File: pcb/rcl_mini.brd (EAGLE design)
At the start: 160 x 100 mm, 59 parts, among them CN1 USB mini B, Q1 8MHz, Q2 IRLML5203, U1 MCP6002T-I/SN, U2 MCP6002T-I/SN, U3 MCP6002T-I/SN, U4 STM32F100CBT6, U5 MCP73831/OT, U6 MCP1703CB, X1 BAT, X2 TWEEZERS, X3 OLED, X4 SWD

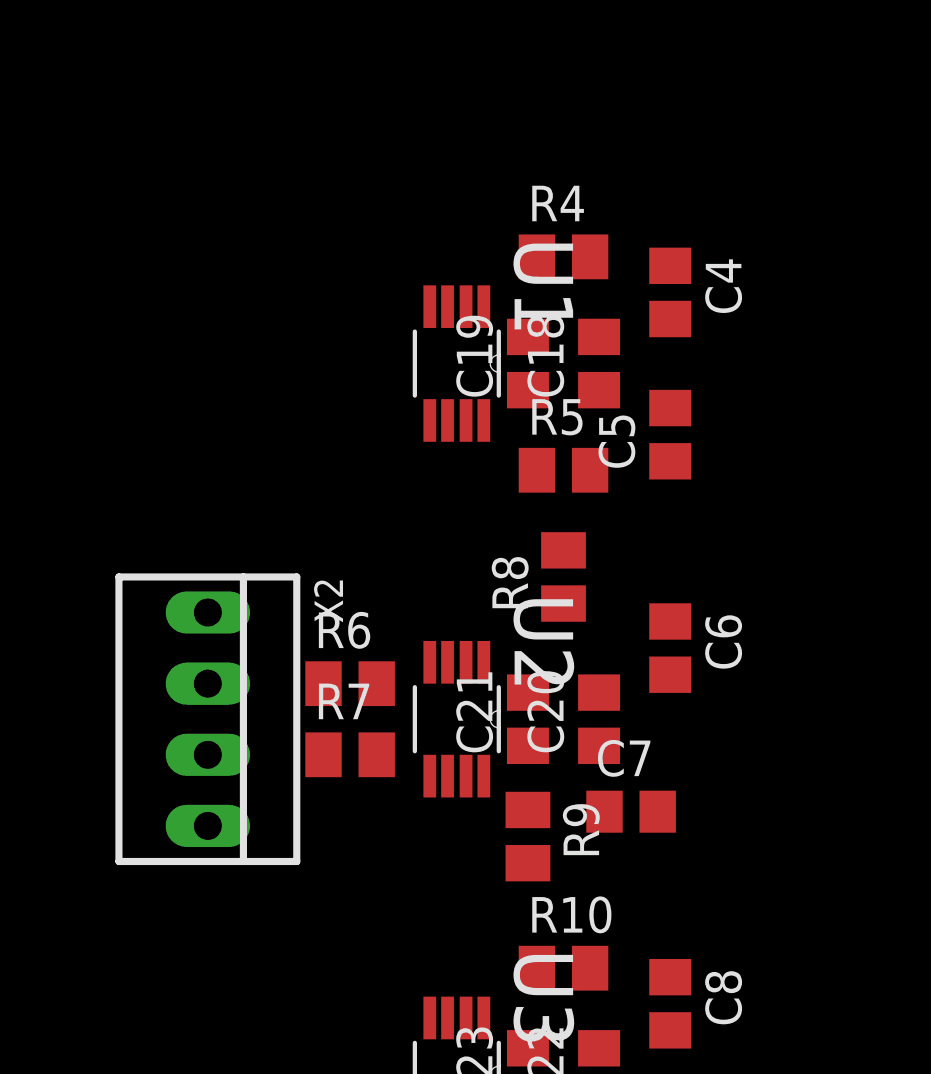
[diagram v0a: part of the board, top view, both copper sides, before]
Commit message: pcb v1.0
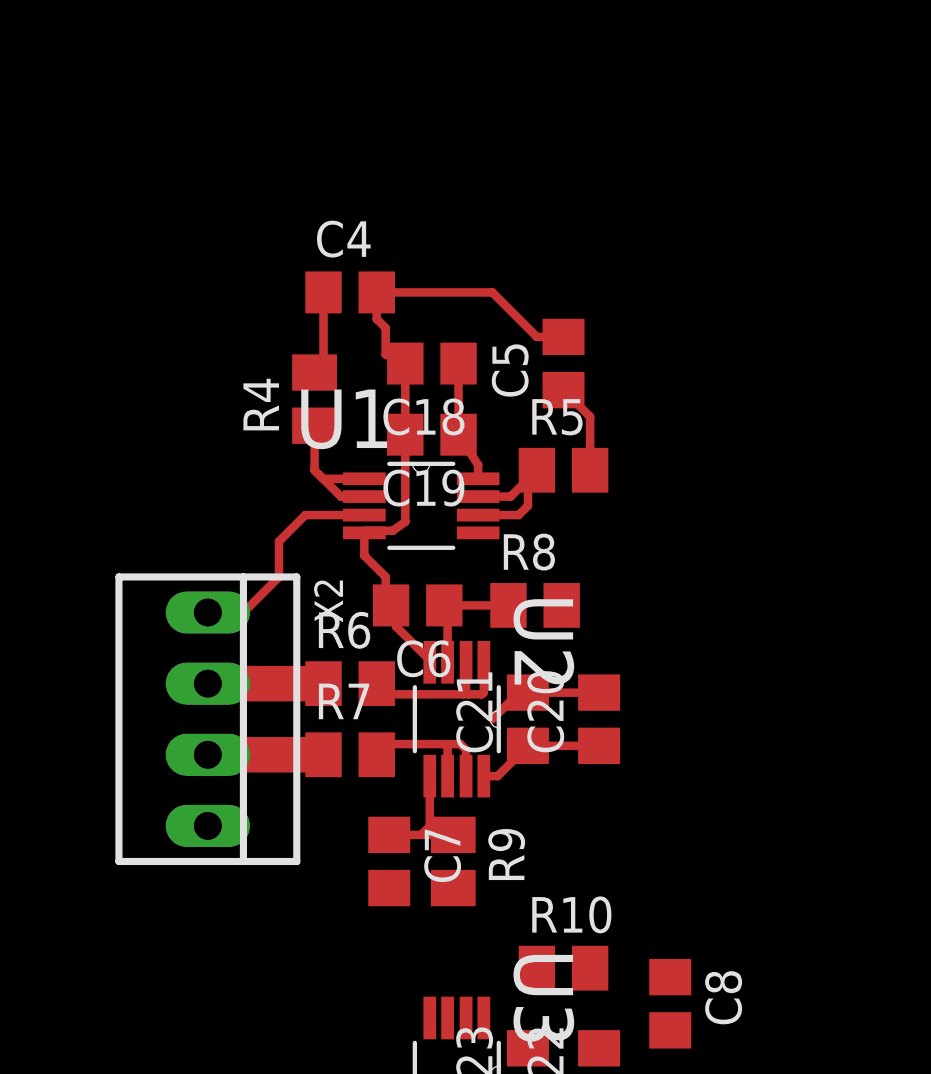
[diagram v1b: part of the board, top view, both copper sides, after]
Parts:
- moved C4 11.4 mm to (15.2, 76.2), turned to 0 degrees
- moved R4 10.2 mm to (14.0, 72.4), turned to 90 degrees
- moved C6 9.14 mm to (17.7, 65.0), turned to 180 degrees
- moved C7 8.82 mm to (16.6, 55.9), turned to 270 degrees
- moved C18 5.97 mm to (18.2, 73.7), turned to 180 degrees
- moved U1 5.24 mm to (17.8, 68.6), turned to 0 degrees
- moved C5 4.58 mm to (22.9, 73.7)
- moved C19 4.27 mm to (18.2, 71.1), turned to 180 degrees
- moved R9 2.81 mm to (18.9, 55.9)
- moved R8 1.44 mm to (21.8, 65.0), turned to 0 degrees
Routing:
- net GND: track 0.00 -> 27.5 mm
- net VCC_OPAMP: track 0.00 -> 8.89 mm
- net LPOT: track 0.00 -> 7.77 mm
- net LCUR2: track 0.00 -> 6.21 mm
- net N$10: track 0.00 -> 5.80 mm
- net N$6: track 0.00 -> 5.66 mm
- net HCUR2: track 0.00 -> 5.54 mm
- net LCUR: track 0.00 -> 5.40 mm
- net N$16: track 0.00 -> 4.51 mm
- net N$11: track 0.00 -> 4.37 mm
- net HCUR: track 0.00 -> 4.13 mm
- net PA2: track 0.00 -> 3.25 mm
- net PA1: track 0.00 -> 2.99 mm
